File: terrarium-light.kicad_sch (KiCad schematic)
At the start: 37 parts, among them J1 USB_C_Receptacle_USB2.0_14P, Q1 UMH3N, U1 CH340C, U2 AL8860WT, U3 AL8860WT

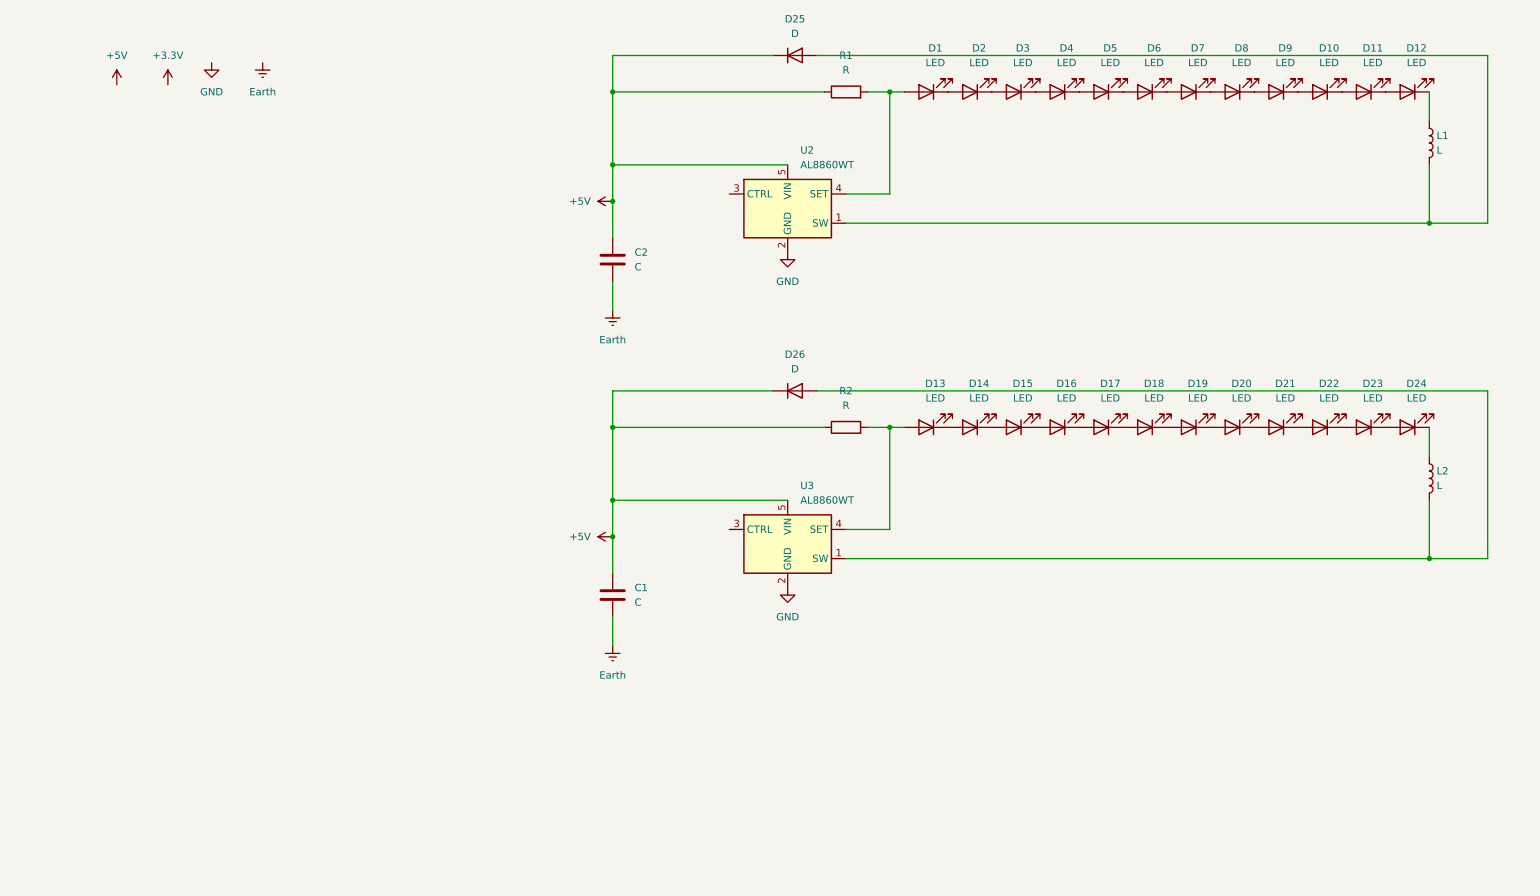
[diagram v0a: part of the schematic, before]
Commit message: updates
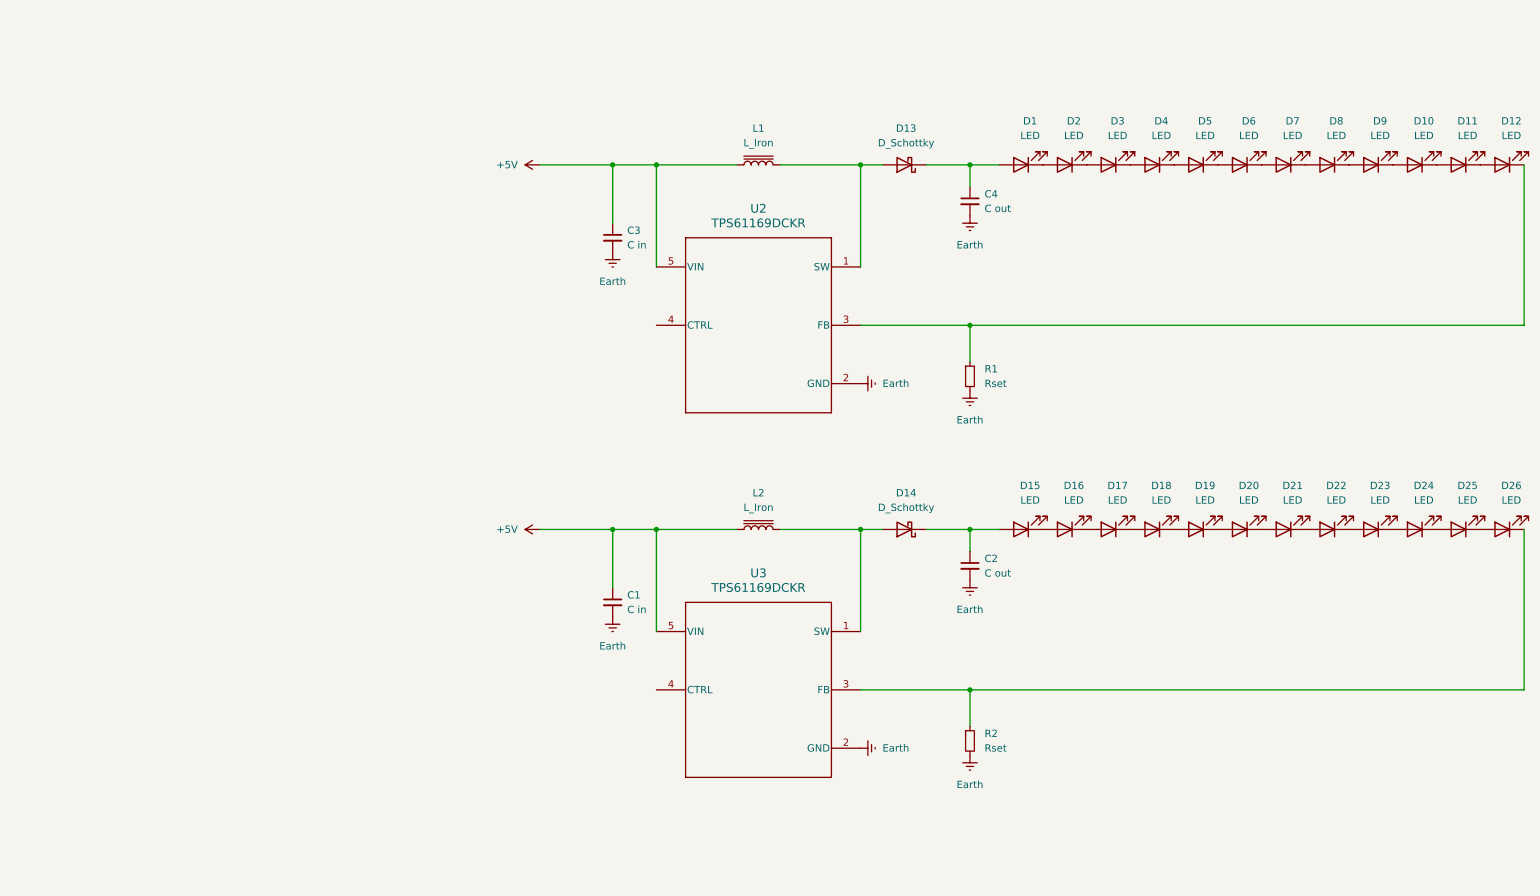
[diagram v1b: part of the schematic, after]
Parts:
- removed C1, C2: C, symbol Device:C
- removed D13, D14: LED, symbol Device:LED
- removed D25, D26: D, symbol Device:D
- removed L1, L2: L, symbol Device:L
- removed R1, R2: R, symbol Device:R
- removed U2, U3: AL8860WT, Package_TO_SOT_SMD:TSOT-23-5, symbol Driver_LED:AL8860WT
- added C1, C3: C in, symbol Device:C_Small
- added C2, C4: C out, symbol Device:C_Small
- added D13, D14: D_Schottky, symbol Device:D_Schottky
- added D25, D26: LED, symbol Device:LED
- added L1, L2: L_Iron, symbol Device:L_Iron
- added R1, R2: Rset, symbol Device:R_Small
- added U2, U3: TPS61169DCKR, DCK0005A_N, symbol TPS61169DCKR:TPS61169DCKR
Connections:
- net +5V: now also C1.1, C3.1, L1.1, L2.1, U2.5 (VIN), U3.5 (VIN)
- net Earth: now also C1.2, C2.2, C3.2, C4.2, R1.2, R2.2, U2.2 (GND), U3.2 (GND)
- net at D12.1 (K): now also R1.1, U2.3 (FB)
- net at D24.1 (K): now also D25.2 (A)
- net at D1.2 (A): now also C4.1, D13.1 (K)
- net at D15.2 (A): now also C2.1, D14.1 (K)
- new net: D14.2 (A), L2.2, U3.1 (SW)
- new net: D26.1 (K), R2.1, U3.3 (FB)
- new net: D25.1 (K), D26.2 (A)
- new net: D13.2 (A), L1.2, U2.1 (SW)
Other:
- moved on the sheet: D1, D10, D11, D12, D2, D3, D4, D5, D6, D7, D8, D9

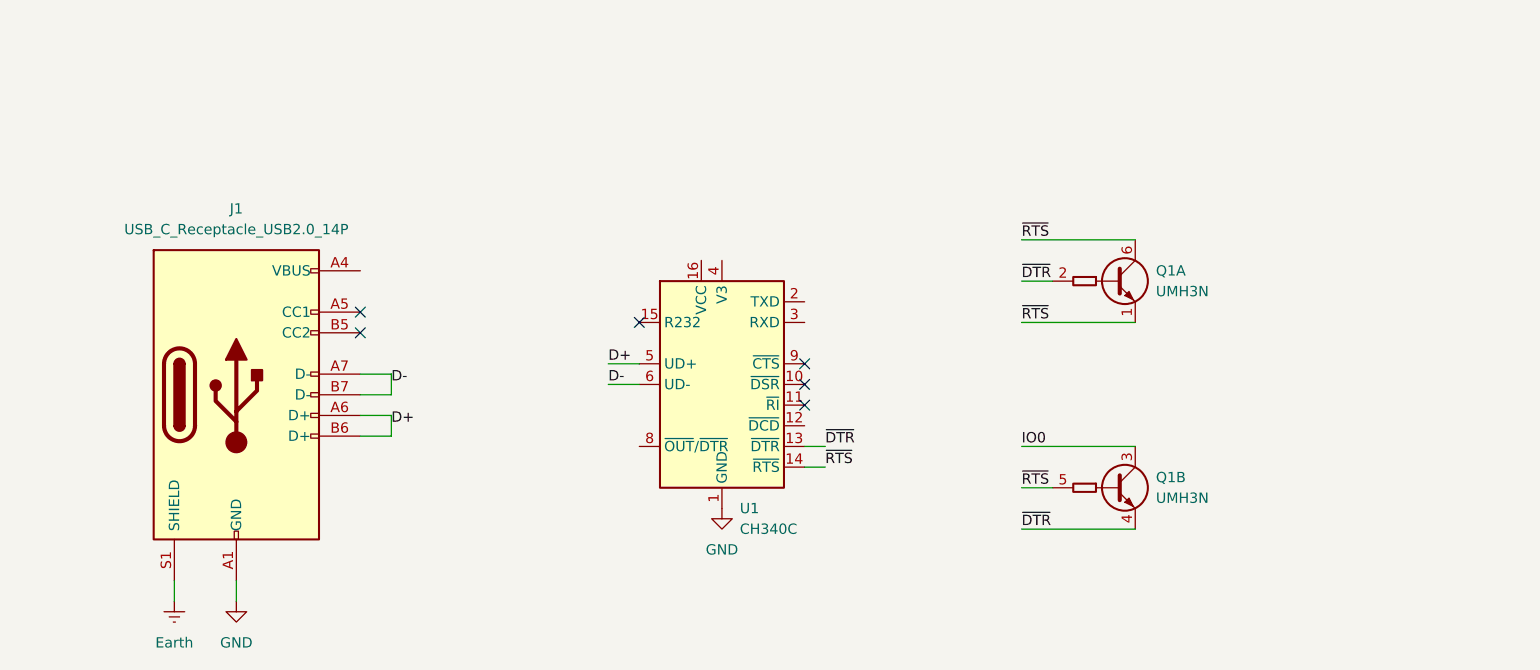
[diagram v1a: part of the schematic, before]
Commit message: CH340C seems good
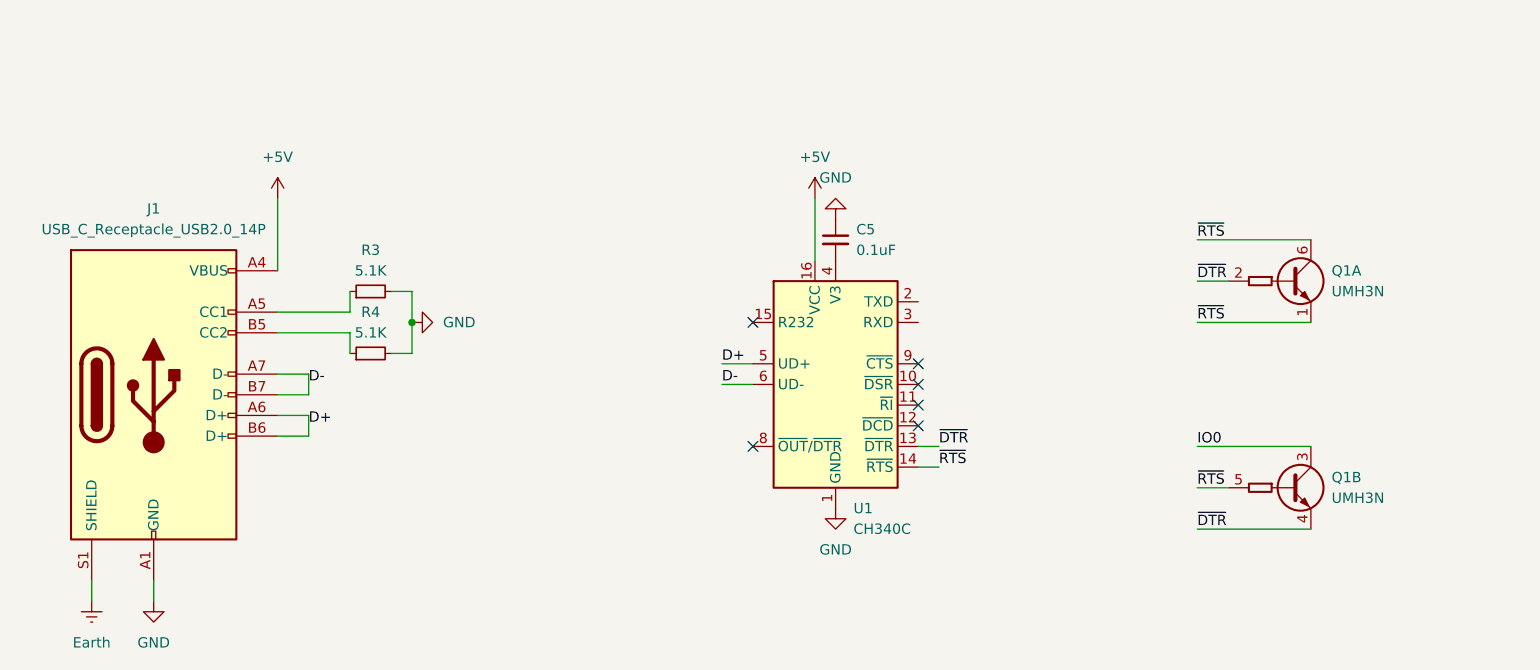
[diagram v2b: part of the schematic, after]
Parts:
- added C5: 0.1uF, symbol Device:C_Small
- added R3, R4: 5.1K, symbol Device:R_Small
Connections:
- net +5V: now also J1.A4 (VBUS), J1.A9 (VBUS), J1.B4 (VBUS), J1.B9 (VBUS), U1.16 (VCC)
- net GND: now also C5.1, R3.2, R4.2
- net at U1.4 (V3): now also C5.2
- net at J1.A5 (CC1): now also R3.1
- net at J1.B5 (CC2): now also R4.1
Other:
- moved on the sheet: J1, Q1A, Q1B, U1

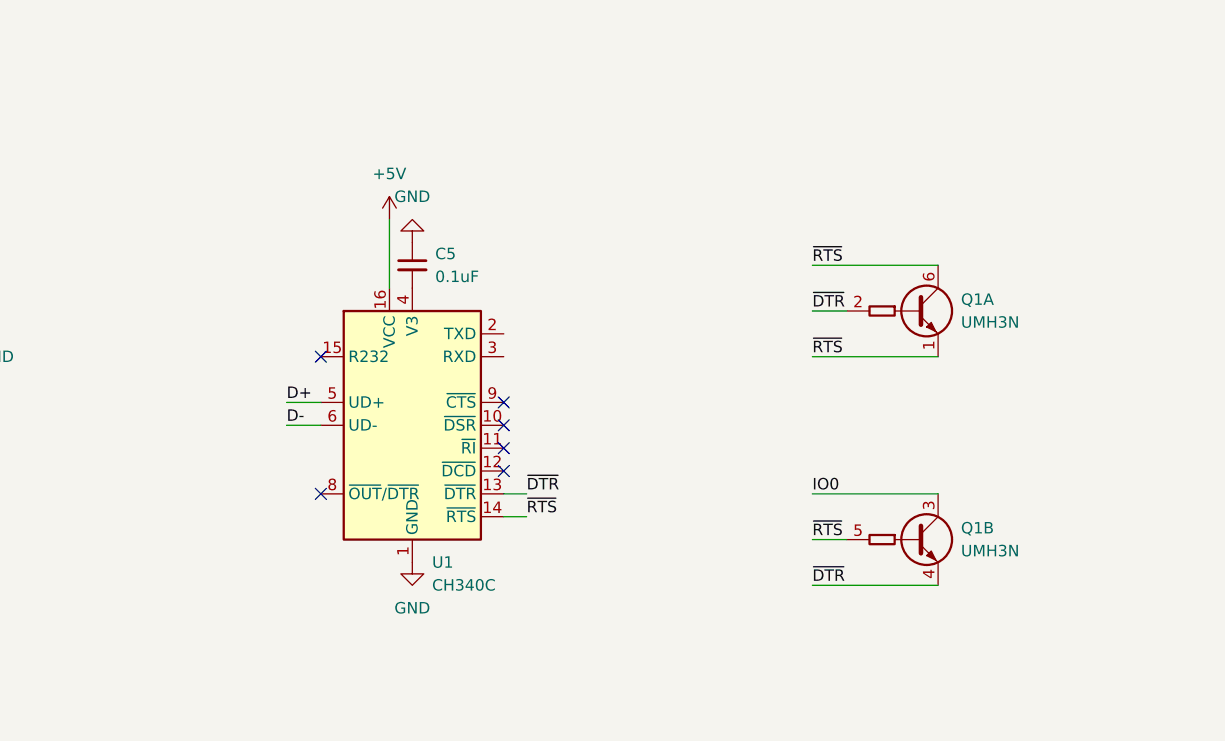
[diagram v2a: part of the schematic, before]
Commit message: updates
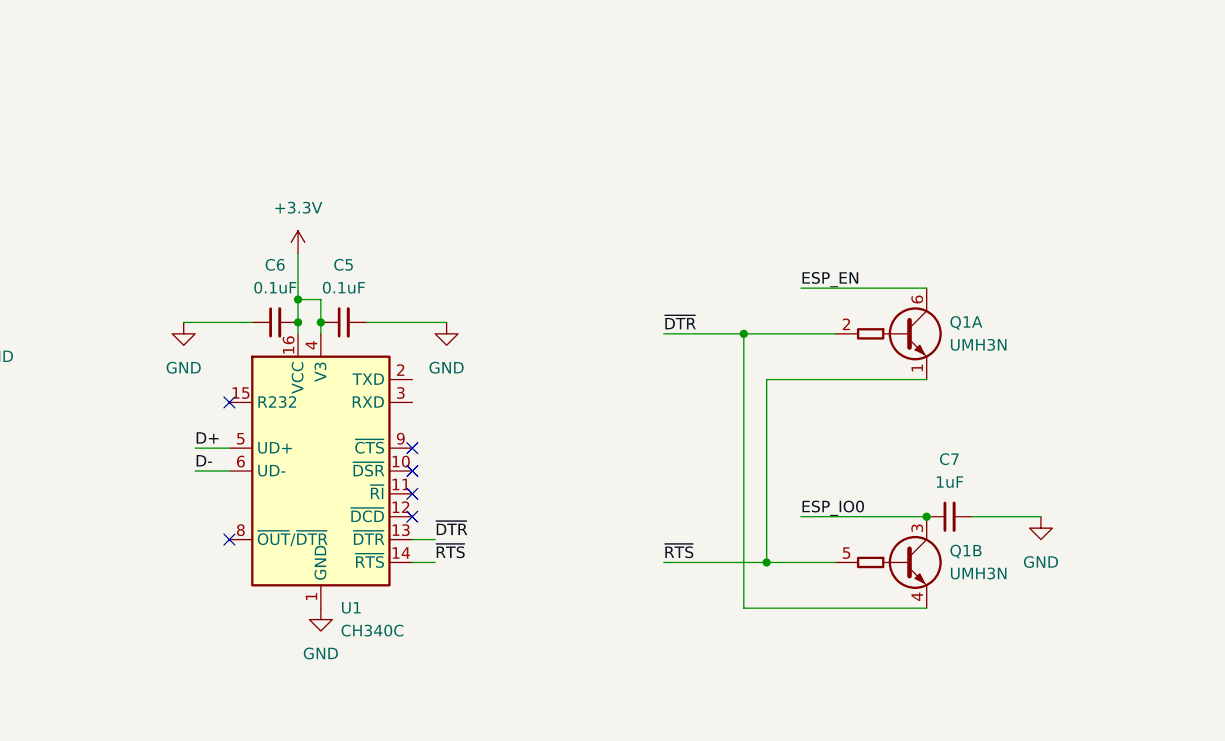
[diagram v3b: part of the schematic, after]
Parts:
- added C6: 0.1uF, symbol Device:C_Small
- added C7: 1uF, symbol Device:C_Small
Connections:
- net +5V: no longer U1.16 (VCC)
- net GND: now also C5.2, C6.1, C7.2; no longer C5.1
- net ~{RTS}: no longer Q1.6 (C1)
- net +3.3V: now reaches U1.4 (V3)
- net +3.3V: now also C5.1, U1.16 (VCC), C6.2; no longer C5.2
- net IO0 renamed ESP_IO0
- net ESP_IO0: now also C7.1
- new net ESP_EN: Q1.6 (C1)
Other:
- moved on the sheet: C5, Q1A, Q1B, U1
